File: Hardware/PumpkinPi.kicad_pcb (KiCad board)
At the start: 4 copper layers, 16 parts, among them J1 Conn_01x02_Male, J2 Conn_01x04, J3 0475710001, U1 F1C100s, U2 TPS717xx, U3 TPS717xx, U4 TPS717xx, Y1 Crystal_GND24

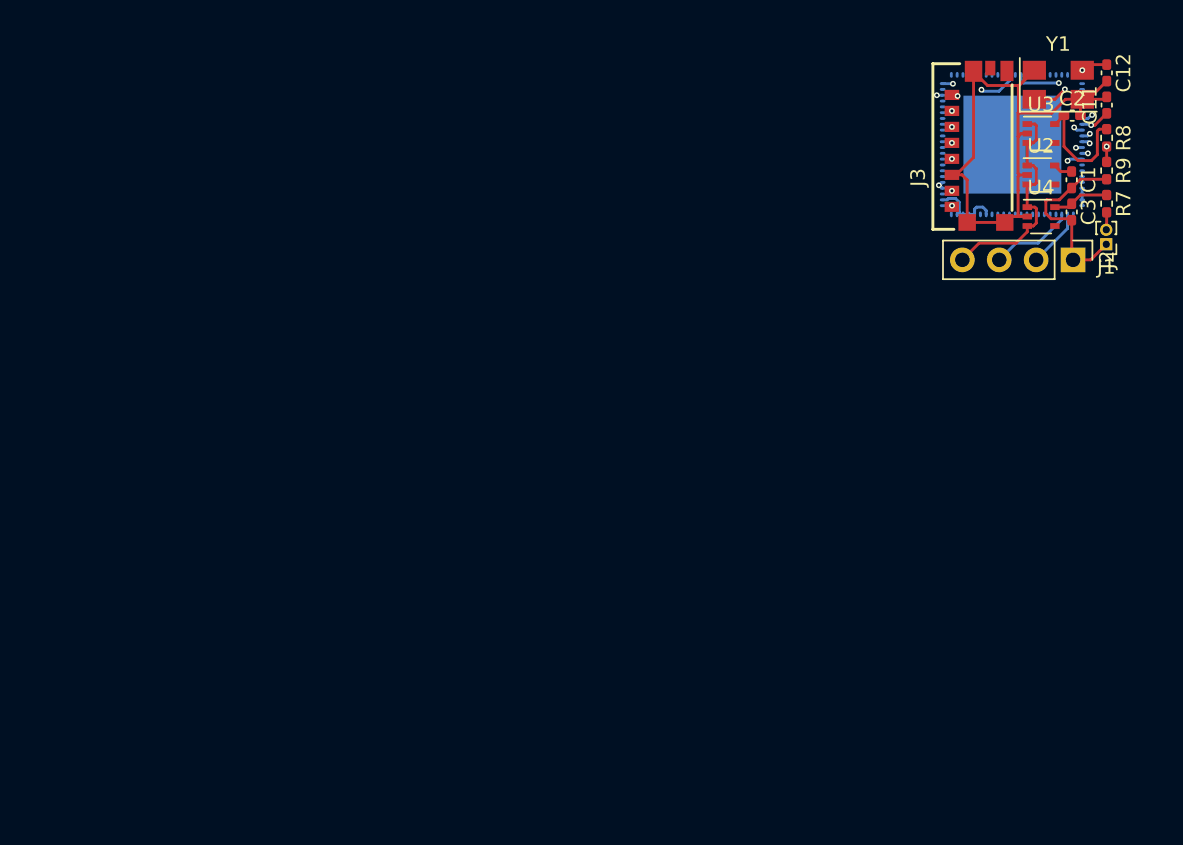
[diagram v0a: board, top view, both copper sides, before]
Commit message: minor changes
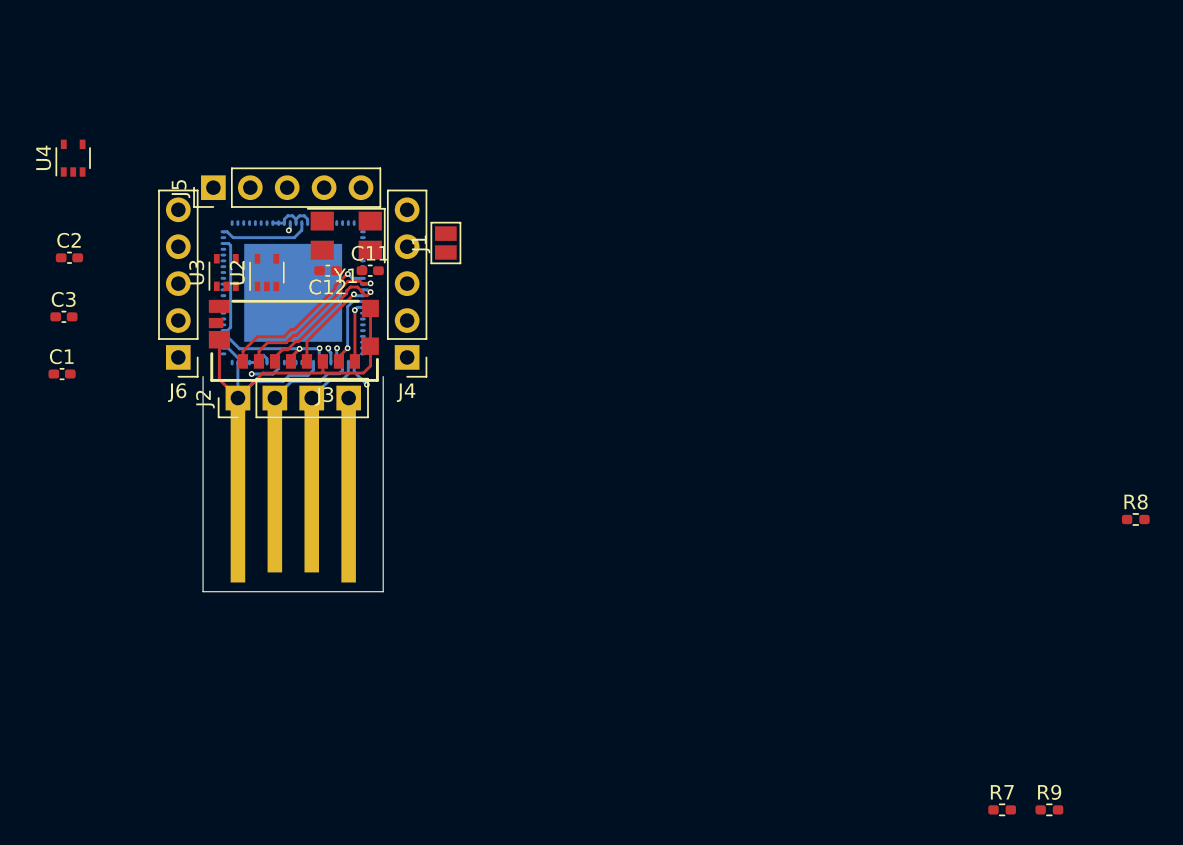
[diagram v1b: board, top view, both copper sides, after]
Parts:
- added J4: Conn_01x05, Connector_PinHeader_2.54mm:PinHeader_1x05_P2.54mm_Vertical, F.Cu at (114.0, 98.7)
- added J5: Conn_01x05, Connector_PinHeader_2.54mm:PinHeader_1x05_P2.54mm_Vertical, F.Cu at (100.7, 87.0)
- added J6: Conn_01x05, Connector_PinHeader_2.54mm:PinHeader_1x05_P2.54mm_Vertical, F.Cu at (98.3, 98.7)
- J1: footprint Connector_PinHeader_1.00mm:PinHeader_1x02_P1.00mm_Vertical -> Jumper:SolderJumper-2_P1.3mm_Open_Pad1.0x1.5mm
- J2: footprint Connector_PinHeader_2.54mm:PinHeader_1x04_P2.54mm_Vertical -> PumpkinPi:USB_PCB
- moved C1 70.8 mm to (90.3, 99.8), turned to 0 degrees
- moved C3 69.7 mm to (90.4, 95.9), turned to 0 degrees
- moved C2 69.7 mm to (90.8, 91.8)
- moved U4 66.7 mm to (91.1, 85.0), turned to 90 degrees
- moved J2 58.3 mm to (102.4, 101.5), turned to 90 degrees
- moved U3 56.9 mm to (101.6, 92.8), turned to 90 degrees
- moved C12 55.3 mm to (108.6, 92.7), turned to 180 degrees
- moved U2 53.7 mm to (104.4, 92.8), turned to 90 degrees
- moved C11 52.0 mm to (111.5, 92.7), turned to 0 degrees
- moved U1 50.5 mm to (106.2, 94.2)
- moved Y1 50.1 mm to (109.9, 90.3), turned to 180 degrees
- moved J3 48.5 mm to (106.3, 97.5), turned to 180 degrees
- moved J1 45.4 mm to (116.7, 90.8), turned to 90 degrees
- moved R9 44.2 mm to (158.2, 129.8), turned to 0 degrees
- moved R7 42.3 mm to (155.0, 129.8), turned to 0 degrees
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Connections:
- J2 pad 2: /USB_DM -> /USB_P
- J2 pad 3: /USB_DP -> /USB_N
- U1 pad 13: (no net) -> /PD7
- U1 pad 14: (no net) -> /PD8
- U1 pad 15: (no net) -> /PD9
- U1 pad 16: (no net) -> /PD10
- U1 pad 37: (no net) -> /SDA
- U1 pad 38: (no net) -> /SCL
- U1 pad 48: (no net) -> /TX
- U1 pad 49: (no net) -> /RX
- U1 pad 59: (no net) -> /SPI_CLK
- U1 pad 60: (no net) -> /SPI_CS
- U1 pad 61: (no net) -> /SPI_MISO
- U1 pad 62: (no net) -> /SPI_MOSI
- U1 pad 68: /USB_DM -> /USB_N
- U1 pad 69: /USB_DP -> /USB_P
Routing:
- net GND: track 63.4 -> 34.0 mm
- net /SVREF: track 18.0 -> 0.54 mm, vias 2 -> 1
- net /USB_VBUS: track 15.9 -> 0.00 mm
- net /CLKP: track 8.38 -> 0.00 mm, vias 2 -> 0
- net /SD0_D1: track 11.4 -> 4.16 mm, vias 2 -> 1
- net /SD0_D0: track 11.6 -> 5.22 mm, vias 2 -> 1
- net /CLKN: track 5.99 -> 0.00 mm, vias 2 -> 0
- net /USB_P: track 0.00 -> 5.98 mm
- net +1V1: track 13.3 -> 7.33 mm, vias 2 -> 1
- net +3V3: track 12.3 -> 18.2 mm
- net /USB_DP: track 5.80 -> 0.00 mm
- net /USB_DM: track 4.03 -> 0.00 mm
- net /USB_N: track 0.00 -> 3.98 mm
- net /SD0_CLK: track 9.45 -> 6.61 mm, vias 2 -> 1
- net +2V5: track 8.19 -> 5.98 mm, vias 0 -> 1
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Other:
- board outline added: 12.4 x 14.8 mm
